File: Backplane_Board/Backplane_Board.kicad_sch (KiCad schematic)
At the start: 14 parts, among them J17 Conn_01x02_Pin

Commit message: backup before heavy revtion
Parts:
- removed C11, C12, C13: C_Polarized_US, symbol Device:C_Polarized_US
- removed D10: ZPDxx, Diode_THT:D_DO-35_SOD27_P10.16mm_Horizontal, symbol Diode:ZPDxx
- removed D11: LED, symbol Device:LED
- removed R19, R21, R22: R, symbol Device:R
- removed R20: 3K, symbol Device:R
- removed U1, U3: ~, symbol PKJ7213WPI:PKJ7213WPI
- added D1: LED, symbol Device:LED
- added D2: D, symbol Device:D
- added Q1: Q_NMOS_DGS, symbol Device:Q_NMOS_DGS
- added R5: R, symbol Device:R
- added U1: TCR2EE11, Package_TO_SOT_SMD:SOT-553, symbol Regulator_Linear:TCR2EE11
- C4, C5: value C_Polarized_US -> 330uF
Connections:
- net 60V: now also Q1.1 (D); no longer J17.1 (Pin_1)
- net GND: now also R5.2, U1.2 (GND)
- new net: D2.1 (K), U1.3 (VIN)
- new net: D2.2 (A), J17.1 (Pin_1), Q1.3 (S)
- new net: D1.1 (K), R5.1
- new net: D1.2 (A), Q1.2 (G), U1.4 (VOUT)
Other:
- note added: "Reverse input voltage protection. I did it this way, insted of using a p-chanle becuse will be having varing voltage levels (also need a status LED, so have the ragulator anyways) (to protect the ragulator, we can use a scotty diode)"
- note removed: "indivdual fuses?"
- moved on the sheet: C4, C5

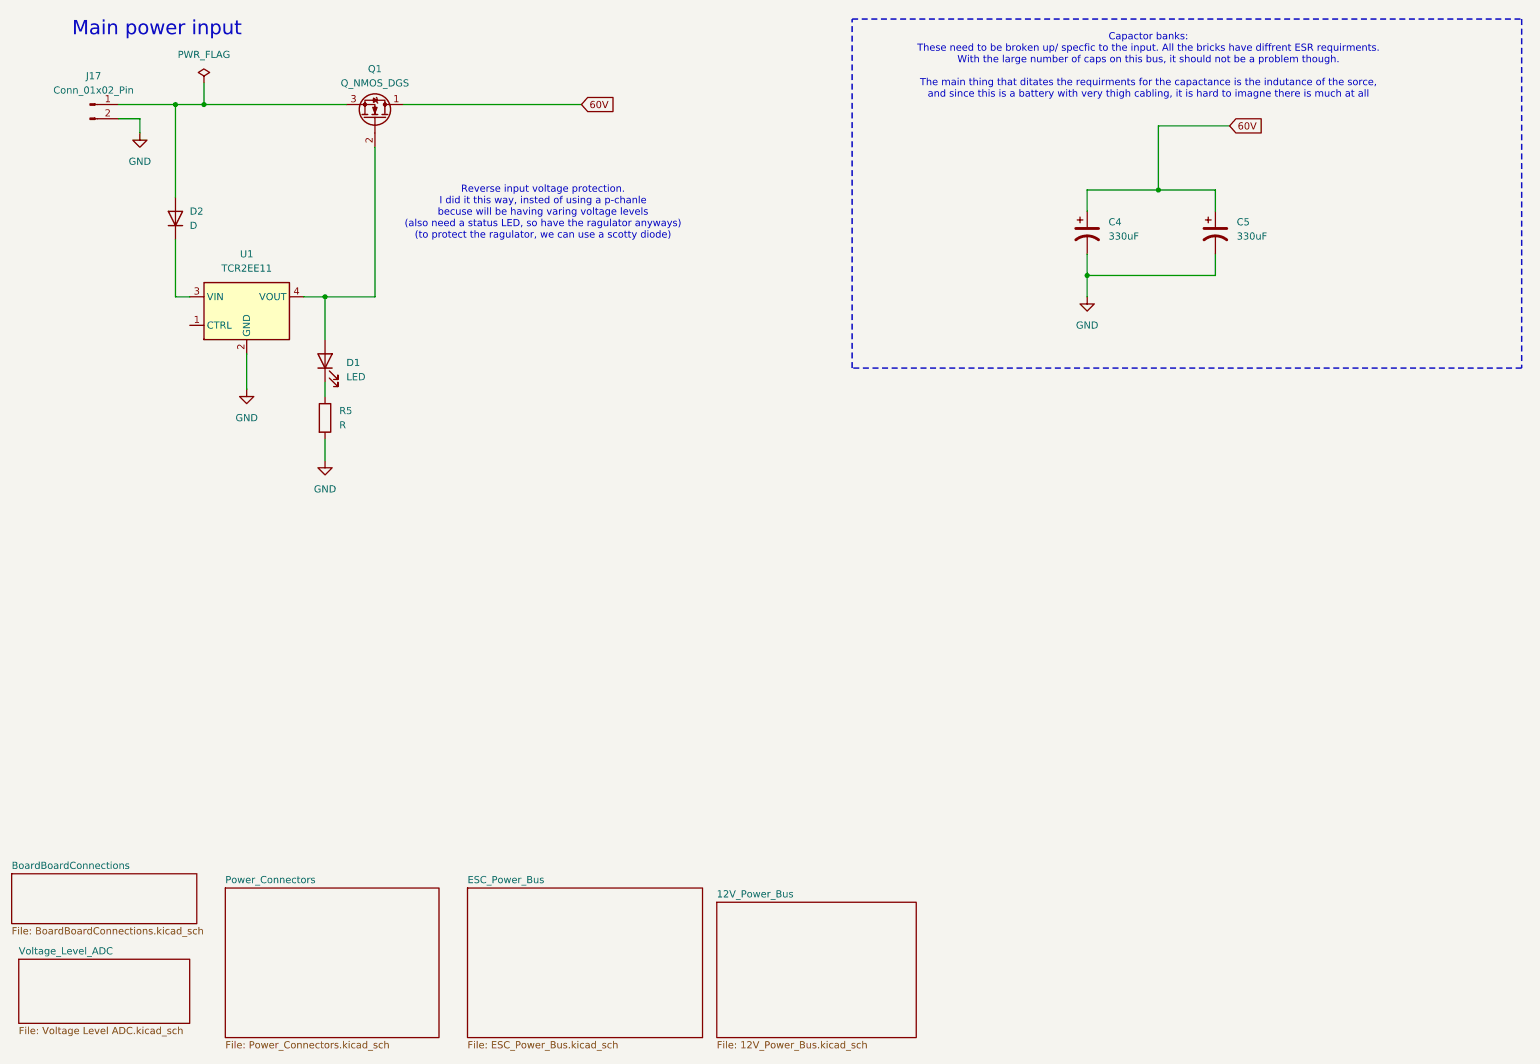
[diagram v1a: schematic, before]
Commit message: back plane board ready for review
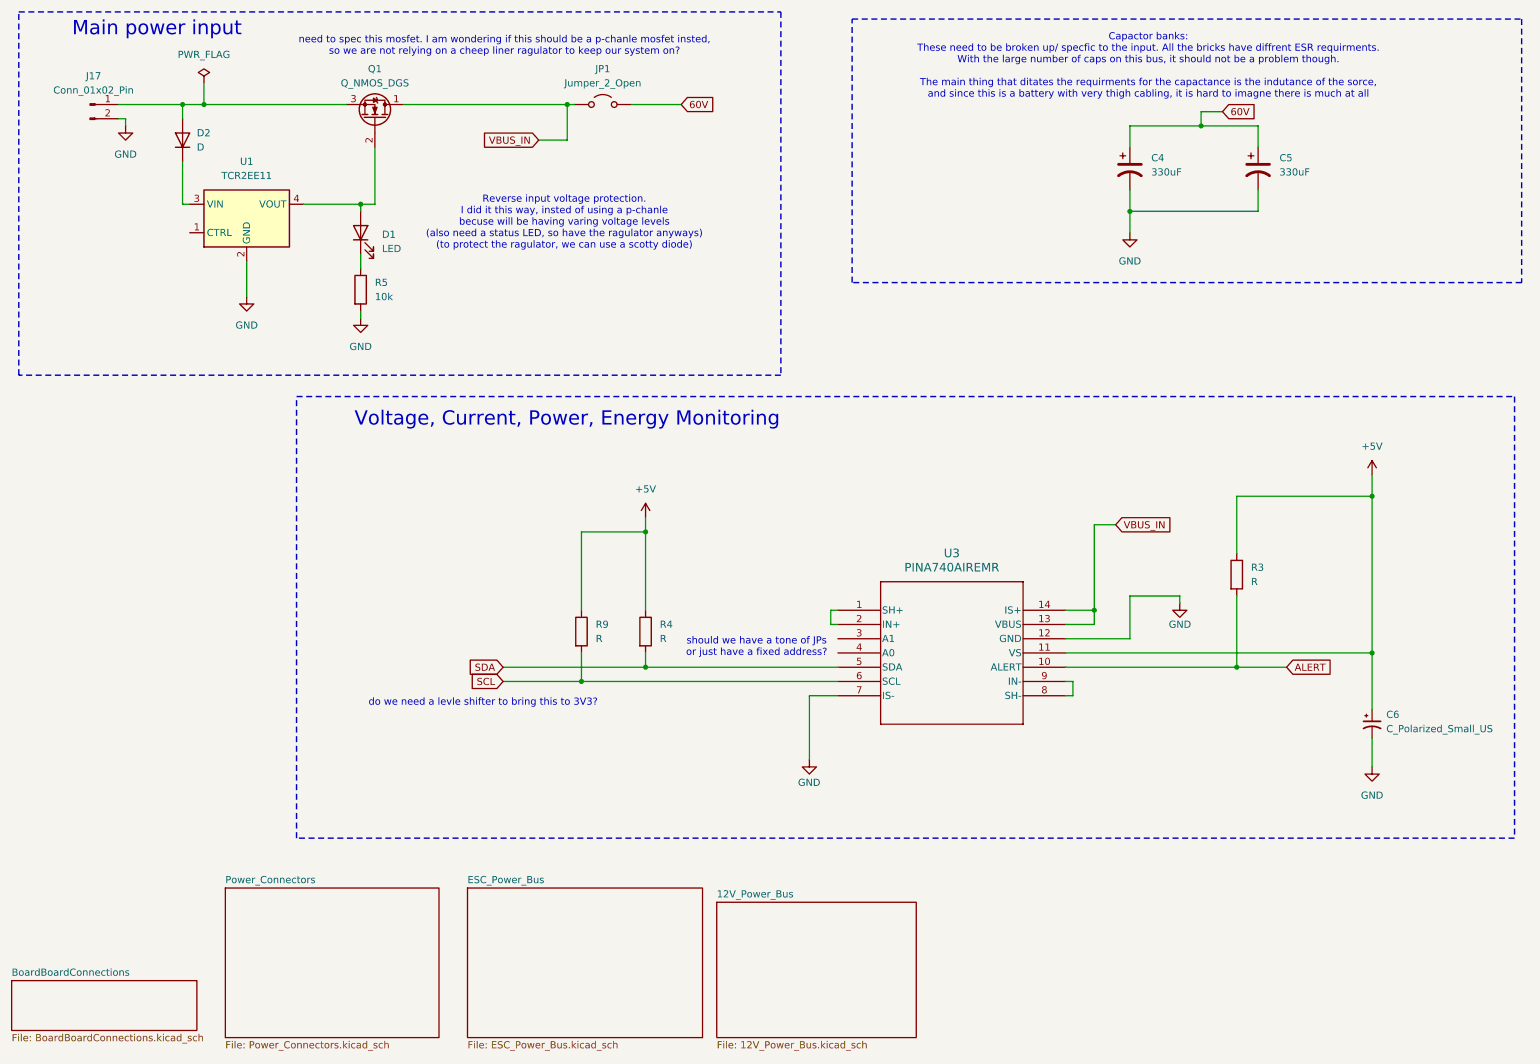
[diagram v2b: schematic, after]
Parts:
- added C6: C_Polarized_Small_US, symbol Device:C_Polarized_Small_US
- added JP1: Jumper_2_Open, symbol Jumper:Jumper_2_Open
- added R3, R4, R9: R, symbol Device:R
- added U3: PINA740AIREMR, VQFN14_REM_TEX, symbol INA740BIREMR:PINA740AIREMR
- R5: value R -> 10k
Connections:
- net 60V: now also JP1.2 (B); no longer Q1.1 (D)
- net GND: now also C6.2, U3.12 (GND), U3.7 (IS-)
- new net: U3.1 (SH+), U3.2 (IN+)
- new net: U3.8 (SH-), U3.9 (IN-)
- new net +5V: C6.1, R3.1, R4.1, R9.1, U3.11 (VS)
- new net ALERT: R3.2, U3.10 (ALERT)
- new net SCL: R9.2, U3.6 (SCL)
- new net SDA: R4.2, U3.5 (SDA)
- new net VBUS_IN: JP1.1 (A), Q1.1 (D), U3.13 (VBUS), U3.14 (IS+)
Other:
- removed sheet Voltage_Level_ADC
- note added: "Voltage, Current, Power, Energy Monitoring"
- note added: "do we need a levle shifter to bring this to 3V3?"
- note added: "need to spec this mosfet. I am wondering if this should be a p-chanle mosfet insted, so we are not relying on a cheep liner ragulator to keep our system on?"
- note added: "should we have a tone of JPs or just have a fixed address?"
- moved on the sheet: C4, C5, D1, D2, R5, U1
